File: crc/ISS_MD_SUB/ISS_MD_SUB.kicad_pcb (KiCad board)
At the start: 2 copper layers, 67.5 x 75 mm, 60 parts, among them J10 Enc, J11 Conn_01x02, J12 Conn_01x02, J13 Conn_01x06, J14 Enc, J15 Conn_01x02, J2 Conn_01x04, J3 Conn_01x04, J4 Conn_01x02, J5 Conn_01x02, J6 Conn_01x10, J7 Conn_01x02, J8 Conn_01x06, J9 Conn_01x10, SW2 SW_DIP_x03, SW3 SW_MEC_5E, SW4 SW_DIP_x03, SW5 SW_MEC_5E, U1 STM32F303K8Tx, U2 STM32F303K8Tx, U3 MCP2561-E-SN, U4 MCP2561-E-SN, U5 NJM2845DL1-33-TE1, U6 NJM2845DL1-33-TE1, Y1 Crystal_GND24_Small, Y2 Crystal_GND24_Small

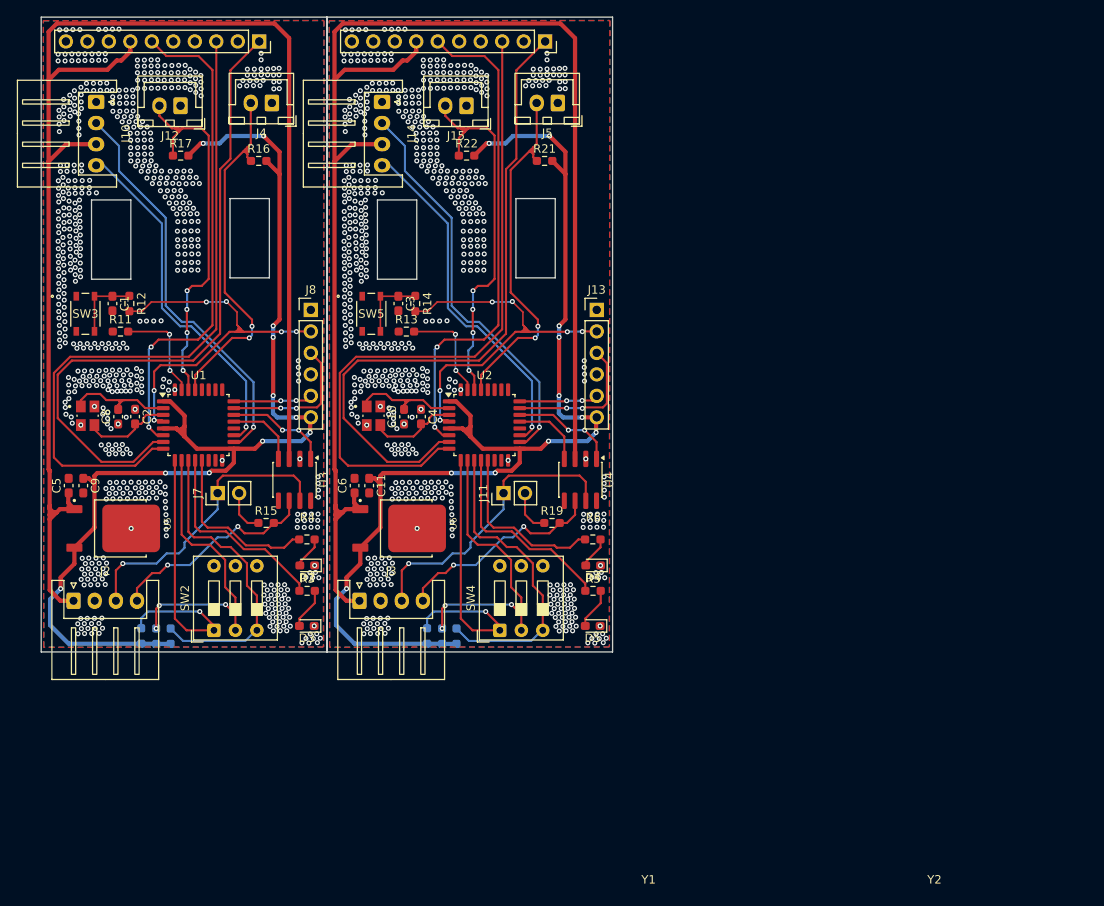
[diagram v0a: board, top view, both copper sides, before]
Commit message: MDSUBのガーバー再生成
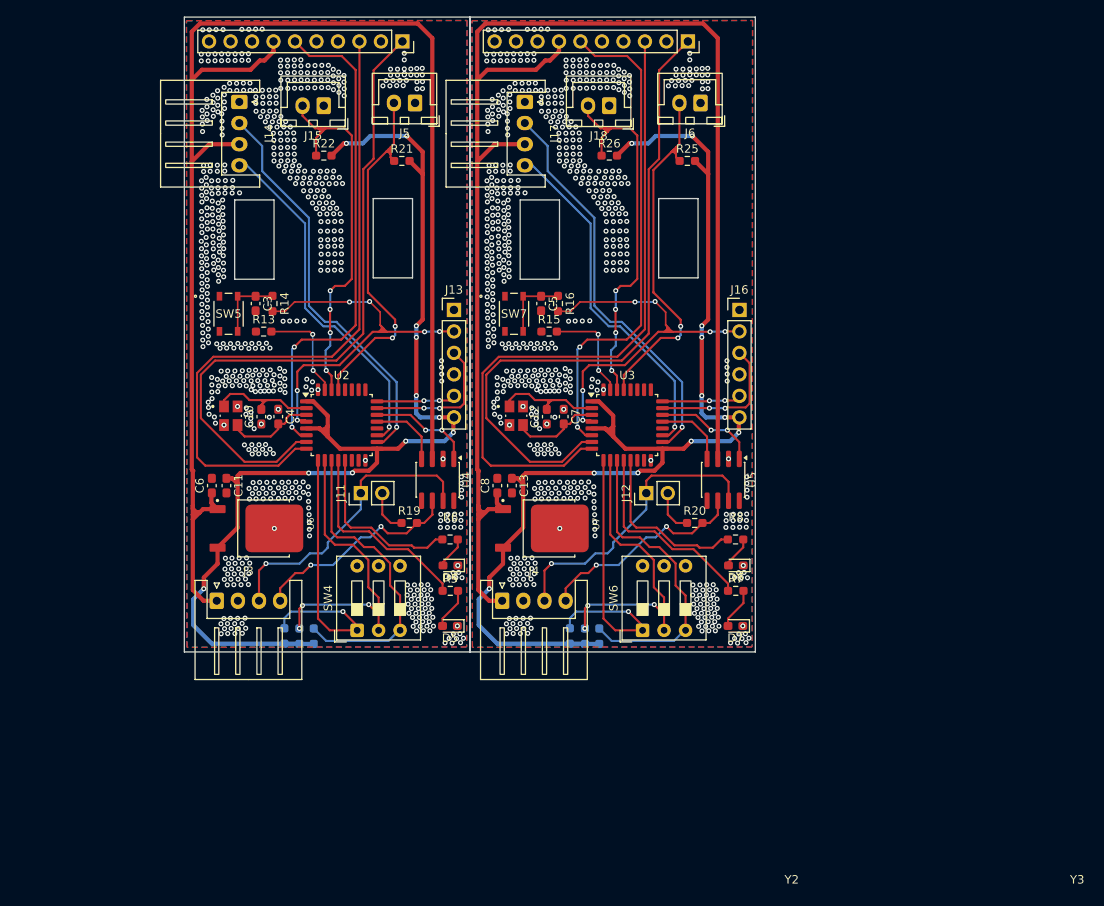
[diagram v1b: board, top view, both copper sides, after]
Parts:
- removed C1, C9: 0.1uF, Capacitor_SMD:C_0603_1608Metric_Pad1.08x0.95mm_HandSolder
- removed C2: 20pF, Capacitor_SMD:C_0603_1608Metric_Pad1.08x0.95mm_HandSolder
- removed the C5 at (112.7, 120.8)
- removed the C8 at (118.5, 112.7)
- removed D2, D3: LED, LED_SMD:LED_0603_1608Metric_Pad1.05x0.95mm_HandSolder
- removed the J10 at (116.0, 75.5)
- removed the J12 at (125.9, 75.9)
- removed J2: Conn_01x04, Connector_JST:JST_XH_S4B-XH-A_1x04_P2.50mm_Horizontal
- removed the J4 at (136.7, 75.6)
- removed the J6 at (135.2, 68.3)
- removed J7: Conn_01x02, Connector_PinHeader_2.54mm:PinHeader_1x02_P2.54mm_Vertical
- removed J8: Conn_01x06, Connector_PinHeader_2.54mm:PinHeader_1x06_P2.54mm_Vertical
- removed the R11 at (118.8, 102.6)
- removed R12: 10k, Resistor_SMD:R_0603_1608Metric_Pad0.98x0.95mm_HandSolder
- removed the R15 at (136.0, 125.2)
- removed the R16 at (135.2, 82.4)
- removed R17, R18, R9: 1k, Resistor_SMD:R_0603_1608Metric_Pad0.98x0.95mm_HandSolder
- removed the R20 at (124.8, 138.6)
- removed R3, R4: 470, Resistor_SMD:R_0603_1608Metric_Pad0.98x0.95mm_HandSolder
- removed SW2: SW_DIP_x03, Button_Switch_THT:SW_DIP_SPSTx03_Slide_9.78x9.8mm_W7.62mm_P2.54mm
- removed SW3: SW_MEC_5E, SKRPABE010:SW4_SKRPABE010_ALPS
- removed U1: STM32F303K8Tx, Package_QFP:LQFP-32_7x7mm_P0.8mm
- removed the U3 at (139.4, 120.1)
- removed the U5 at (118.0, 125.9)
- removed Y1: Crystal_GND24_Small, TSX_3225_25_0000MF10P_C0:XTAL_TSX-3225_25.0000MF10P-C0
- added C10: 20pF, Capacitor_SMD:C_0603_1608Metric_Pad1.08x0.95mm_HandSolder, F.Cu at (135.5, 112.7)
- added C11: 0.1uF, Capacitor_SMD:C_0603_1608Metric_Pad1.08x0.95mm_HandSolder, F.Cu at (131.3, 120.8)
- added C3: 0.1uF, Capacitor_SMD:C_0603_1608Metric_Pad1.08x0.95mm_HandSolder, F.Cu at (134.8, 99.3)
- added C4: 20pF, Capacitor_SMD:C_0603_1608Metric_Pad1.08x0.95mm_HandSolder, F.Cu at (137.5, 112.7)
- added C6: 0.1uF, Capacitor_SMD:C_0603_1608Metric_Pad1.08x0.95mm_HandSolder, F.Cu at (129.6, 120.8)
- added D4: LED, LED_SMD:LED_0603_1608Metric_Pad1.05x0.95mm_HandSolder, F.Cu at (157.8, 130.2)
- added D5: LED, LED_SMD:LED_0603_1608Metric_Pad1.05x0.95mm_HandSolder, F.Cu at (157.8, 137.4)
- added J11: Conn_01x02, Connector_PinHeader_2.54mm:PinHeader_1x02_P2.54mm_Vertical, F.Cu at (147.2, 121.7)
- added J13: Conn_01x06, Connector_PinHeader_2.54mm:PinHeader_1x06_P2.54mm_Vertical, F.Cu at (158.2, 100.0)
- added J14: Enc, Connector_JST:JST_XH_S4B-XH-A_1x04_P2.50mm_Horizontal, F.Cu at (132.9, 75.5)
- added J15: Conn_01x02, Connector_JST:JST_XH_B2B-XH-A_1x02_P2.50mm_Vertical, F.Cu at (142.8, 75.9)
- added J3: Conn_01x04, Connector_JST:JST_XH_S4B-XH-A_1x04_P2.50mm_Horizontal, F.Cu at (130.2, 134.4)
- added J5: Conn_01x02, Connector_JST:JST_XH_B2B-XH-A_1x02_P2.50mm_Vertical, F.Cu at (153.7, 75.6)
- added J9: Conn_01x10, Connector_PinSocket_2.54mm:PinSocket_1x10_P2.54mm_Vertical, F.Cu at (152.2, 68.3)
- added R10: 1k, Resistor_SMD:R_0603_1608Metric_Pad0.98x0.95mm_HandSolder, B.Cu at (140.0, 138.6)
- added R13: 10k, Resistor_SMD:R_0603_1608Metric_Pad0.98x0.95mm_HandSolder, F.Cu at (135.8, 102.6)
- added R14: 10k, Resistor_SMD:R_0603_1608Metric_Pad0.98x0.95mm_HandSolder, F.Cu at (136.8, 99.3)
- added R19: 120, Resistor_SMD:R_0603_1608Metric_Pad0.98x0.95mm_HandSolder, F.Cu at (153.0, 125.2)
- added R21: 1k, Resistor_SMD:R_0603_1608Metric_Pad0.98x0.95mm_HandSolder, F.Cu at (152.1, 82.4)
- added R22: 1k, Resistor_SMD:R_0603_1608Metric_Pad0.98x0.95mm_HandSolder, F.Cu at (142.9, 81.8)
- added R23: 1k, Resistor_SMD:R_0603_1608Metric_Pad0.98x0.95mm_HandSolder, B.Cu at (138.2, 138.6)
- added R24: 1k, Resistor_SMD:R_0603_1608Metric_Pad0.98x0.95mm_HandSolder, B.Cu at (141.7, 138.6)
- added R5: 470, Resistor_SMD:R_0603_1608Metric_Pad0.98x0.95mm_HandSolder, F.Cu at (157.8, 133.2)
- added R6: 470, Resistor_SMD:R_0603_1608Metric_Pad0.98x0.95mm_HandSolder, F.Cu at (157.8, 127.2)
- added SW4: SW_DIP_x03, Button_Switch_THT:SW_DIP_SPSTx03_Slide_9.78x9.8mm_W7.62mm_P2.54mm, F.Cu at (146.8, 137.9)
- added SW5: SW_MEC_5E, SKRPABE010:SW4_SKRPABE010_ALPS, F.Cu at (131.6, 100.5)
- added U2: STM32F303K8Tx, Package_QFP:LQFP-32_7x7mm_P0.8mm, F.Cu at (145.0, 113.7)
- added U4: MCP2561-E-SN, Package_SO:SOIC-8_3.9x4.9mm_P1.27mm, F.Cu at (156.3, 120.1)
- added U6: NJM2845DL1-33-TE1, NJM2845DL1-33-TE1:DPAK228P968X238-4N, F.Cu at (134.9, 125.9)
- added Y2: Crystal_GND24_Small, TSX_3225_25_0000MF10P_C0:XTAL_TSX-3225_25.0000MF10P-C0, F.Cu at (131.9, 112.5)
- moved C12 16.9 mm to (169.2, 112.7)
- moved C13 16.9 mm to (165.1, 120.8)
- moved C5 16.9 mm to (168.6, 99.3)
- moved C7 16.9 mm to (171.2, 112.7)
- moved C8 16.9 mm to (163.4, 120.8)
- moved D6 16.9 mm to (191.6, 130.2)
- moved D7 16.9 mm to (191.5, 137.4)
- moved J10 16.9 mm to (185.9, 68.3)
- moved J12 16.9 mm to (181.0, 121.7)
- moved J16 16.9 mm to (192.0, 100.0)
- moved J17 16.9 mm to (166.6, 75.5)
- moved J18 16.9 mm to (176.6, 75.9)
- moved J4 16.9 mm to (163.9, 134.4)
- moved J6 16.9 mm to (187.4, 75.6)
- moved R11 16.9 mm to (173.7, 138.6)
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- renumbered C10 to C12, C11 to C13, C3 to C5, C4 to C7, C6 to C8, D4 to D6, D5 to D7, J9 to J10, J11 to J12, J13 to J16, J14 to J17, J15 to J18, J3 to J4, J5 to J6, R10 to R11, R13 to R15, R14 to R16, R19 to R20, R21 to R25, R22 to R26, R23 to R27, R24 to R28, R5 to R7, R6 to R8, SW4 to SW6, SW5 to SW7, U2 to U3, U4 to U5, U6 to U7, Y2 to Y3
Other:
- outline, holes or cut-outs redrawn
